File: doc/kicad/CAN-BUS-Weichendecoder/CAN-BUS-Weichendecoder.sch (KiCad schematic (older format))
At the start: 53 parts, among them J1 250-1404, J1001 Conn_01x02_Female, J1003 Conn_01x07_Female, J11 250-1406, J12 Wago 250-1406, J13 Wago 250-1406, J14 Wago 250-1406, J15 Wago 250-1406, J2 250-1404, J22 J22, J23 J22, J3 250-1404, J31 12V DC, J4 250-1404, J41 2604-1102, J5 250-1404, U1 Arduino_Nano, U10 TSR_1-2450, U1001 6N136, U2 ULN2803A, U3 ULN2803A, U4 PCF8574, U5 PCF8574, U6 PCF8574, U7 ULN2803A, U8 ULN2803A, U9 ULN2803A

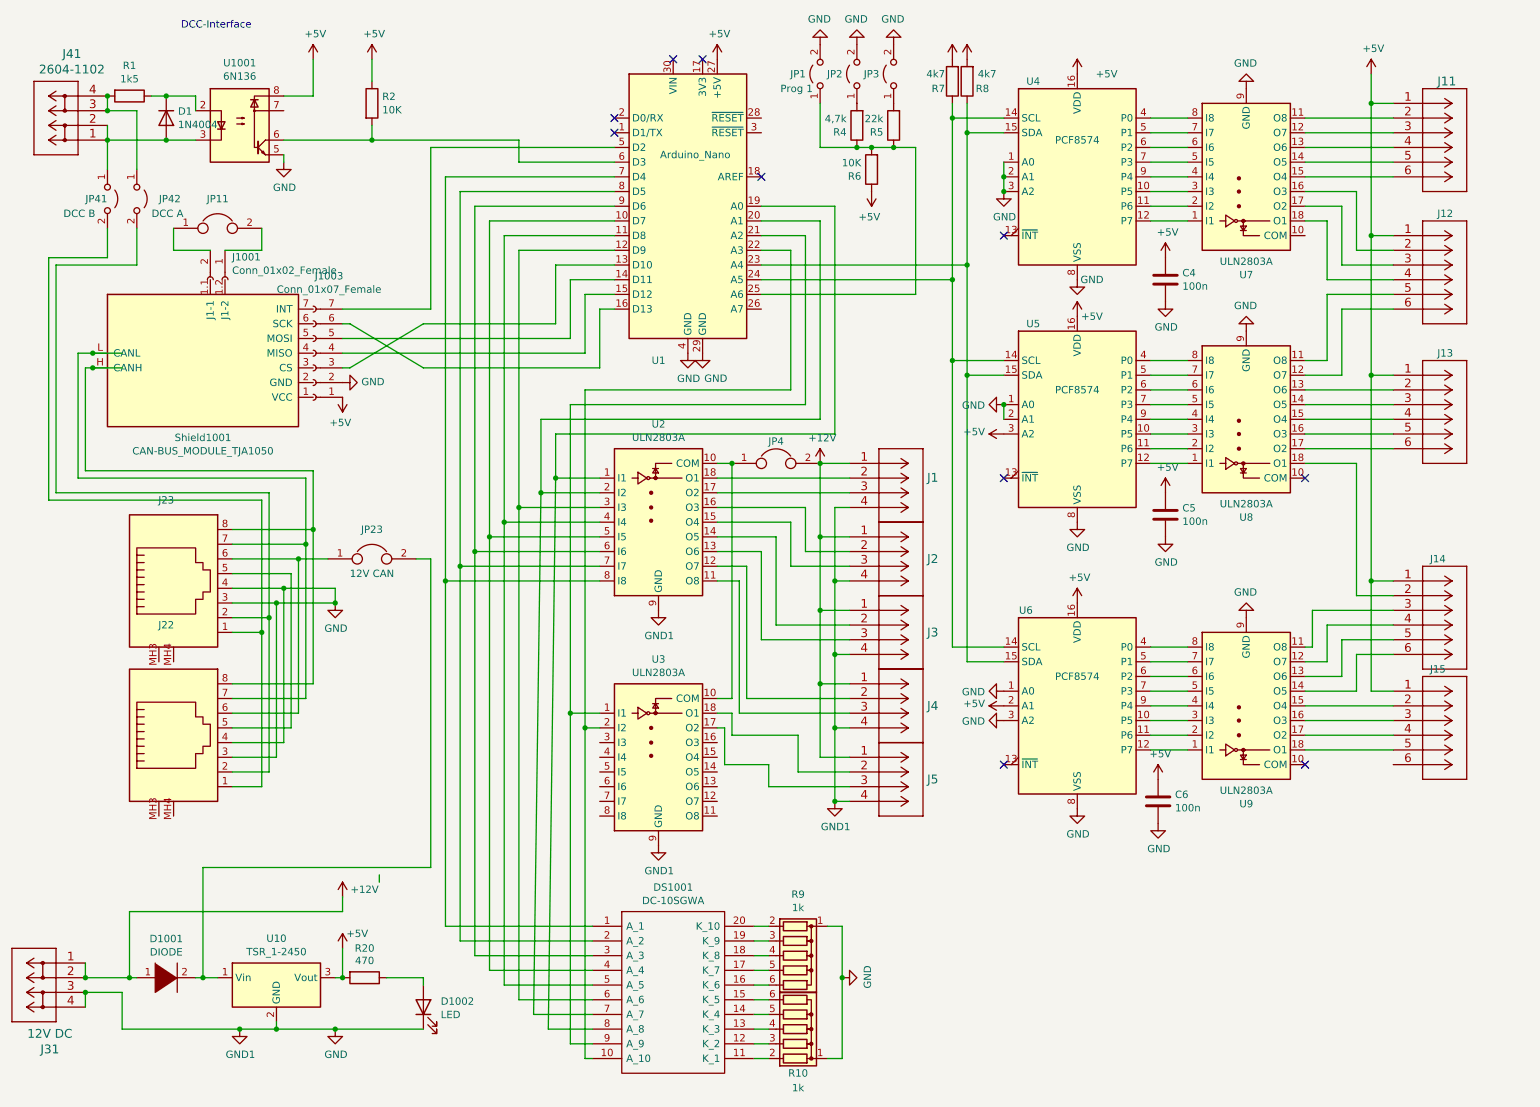
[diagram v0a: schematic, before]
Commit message: verbessert
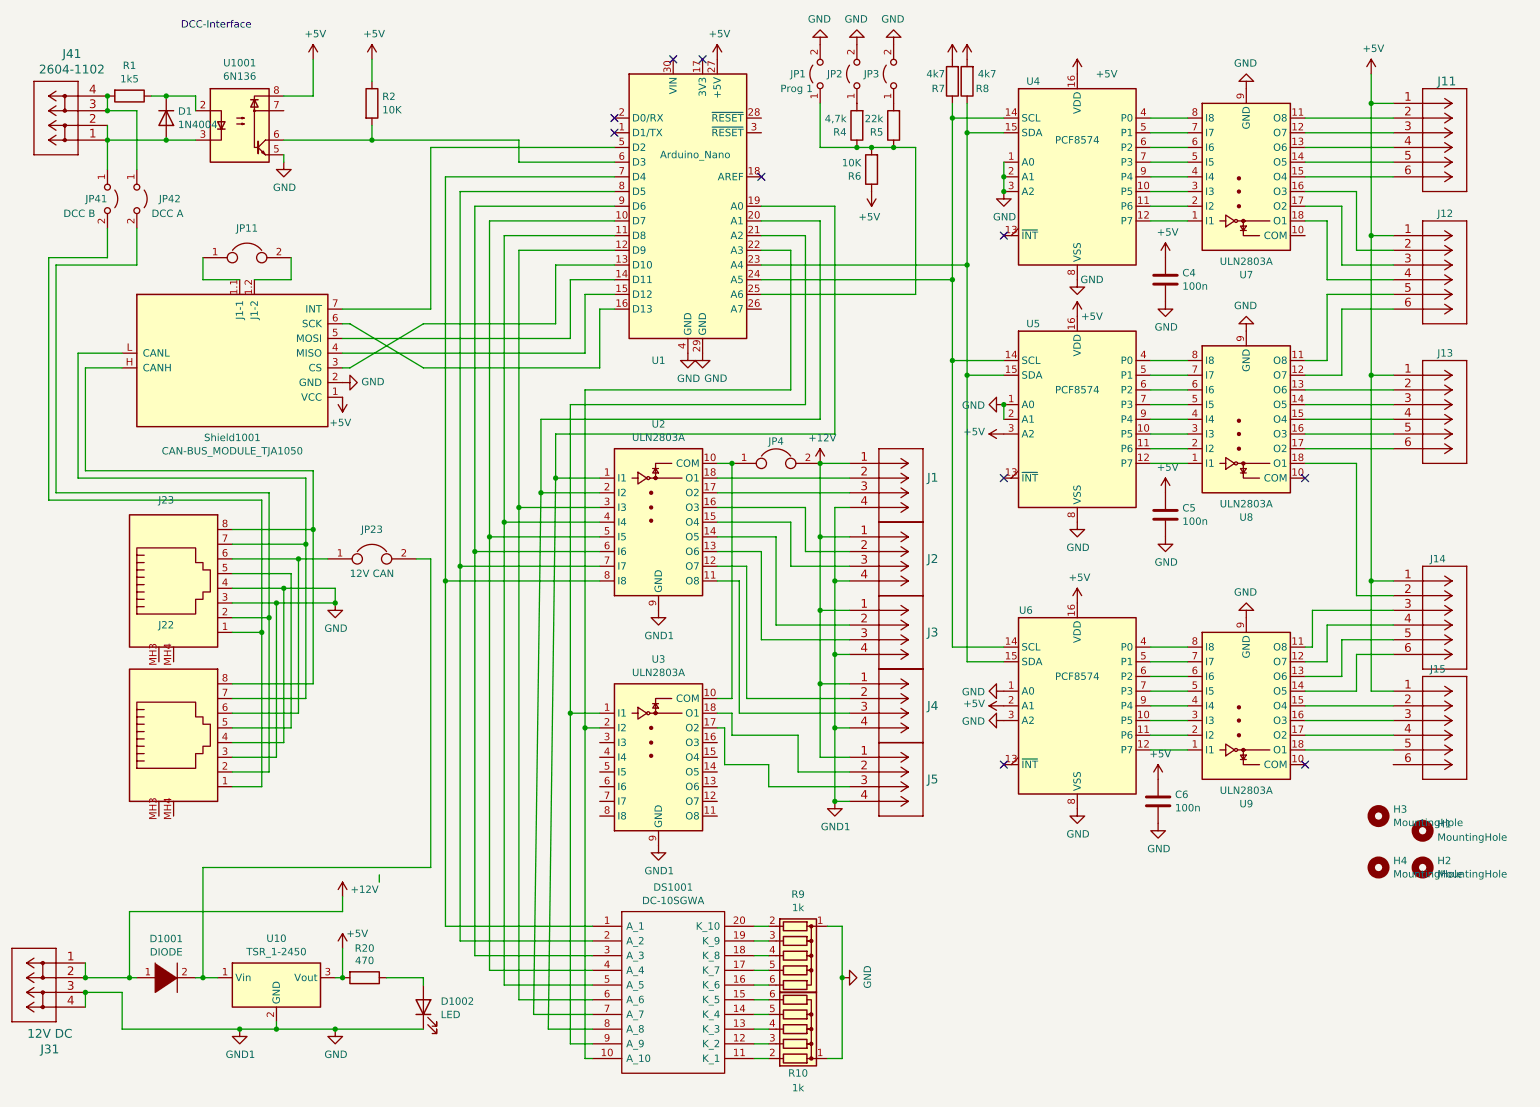
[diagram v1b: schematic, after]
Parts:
- removed J1001: Conn_01x02_Female, Pin_Headers:Pin_Header_Straight_1x02_Pitch2.54mm, symbol Connector:Conn_01x02_Female
- removed J1003: Conn_01x07_Female, Pin_Headers:Pin_Header_Straight_1x07_Pitch2.54mm, symbol Connector:Conn_01x07_Female
- added H1, H2, H3, H4: MountingHole, Mounting_Holes:MountingHole_3.2mm_M3, symbol Mechanical:MountingHole
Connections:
- net +5V: now also Shield1001.1 (VCC)
- net GND: now also Shield1001.2 (GND)
- net at U1.13 (D10): now also Shield1001.3 (CS)
- net at U1.14 (D11): now also Shield1001.5 (MOSI)
- net at U1.15 (D12): now also Shield1001.4 (MISO)
- net at U1.16 (D13): now also Shield1001.6 (SCK)
- net at U1.5 (D2): now also Shield1001.7 (INT)
- net at Shield1001.1.1 (J1-1): now also JP11.1
- net at Shield1001.1.2 (J1-2): now also JP11.2
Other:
- moved on the sheet: JP11, Shield1001
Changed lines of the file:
@@
 L CAN-BUS-MODULE-TJA1050:CAN-BUS_MODULE_TJA1050 Shield1001
 U 1 1 60585225
-P 2000 2650
-F 0 "Shield1001" H 1950 1975 50  0000 C CNN
-F 1 "CAN-BUS_MODULE_TJA1050" H 1950 1884 50  0000 C CNN
-F 2 "CAN-BUS-MODULE:MCP2515_CAN_MODULE_BY0-10" H 2000 2650 50  0001 C CIN
-F 3 "" H 2000 2650 50  0001 C CNN
-	1    2000 2650
+P 2200 2650
+F 0 "Shield1001" H 2150 1975 50  0000 C CNN
+F 1 "CAN-BUS_MODULE_TJA1050" H 2150 1884 50  0000 C CNN
+F 2 "CAN-BUS-MODULE:MCP2515_CAN_MODULE_BY0-10" H 2200 2650 50  0001 C CIN
+F 3 "" H 2200 2650 50  0001 C CNN
+	1    2200 2650
 	1    0    0    -1
 $EndComp
@@
 	2700 5000 2150 5000
 Wire Wire Line
-	1400 2850 1200 2850
+	1400 2850 1150 2850
 Wire Wire Line
 	1150 2850 1150 3550
 Wire Wire Line
-	1400 2750 1200 2750
+	1400 2750 1100 2750
 Wire Wire Line
 	1100 2750 1100 3600
 Wire Wire Line
 	4750 1750 3800 1750
-Connection ~ 1200 2850
-Wire Wire Line
-	1200 2850 1150 2850
-Connection ~ 1200 2750
-$Comp
-L Connector:Conn_01x07_Female J1003
-U 1 1 60962CDF
-P 2700 2750
-F 0 "J1003" H 2592 2225 50  0000 C CNN
-F 1 "Conn_01x07_Female" H 2592 2316 50  0000 C CNN
-F 2 "Pin_Headers:Pin_Header_Straight_1x07_Pitch2.54mm" H 2700 2750 50  0001 C CNN
-F 3 "~" H 2700 2750 50  0001 C CNN
-	1    2700 2750
-	-1   0    0    1
-$EndComp
-Wire Wire Line
-	1100 2750 1200 2750
 $Comp
 L Isolator:6N136 U1001
@@
 	1150 7200 1150 7100
 Connection ~ 1150 7100
-$Comp
-L Connector:Conn_01x02_Female J1001
-U 1 1 61A1EF28
-P 2100 2250
-F 0 "J1001" V 1946 2298 50  0000 L CNN
-F 1 "Conn_01x02_Female" V 2037 2298 50  0000 L CNN
-F 2 "Pin_Headers:Pin_Header_Straight_1x02_Pitch2.54mm" H 2100 2250 50  0001 C CNN
-F 3 "~" H 2100 2250 50  0001 C CNN
-	1    2100 2250
-	0    1    1    0
-$EndComp
-Wire Wire Line
-	1750 1900 1750 2050
-Wire Wire Line
-	1750 2050 2000 2050
-Wire Wire Line
-	2100 2050 2350 2050
-Wire Wire Line
-	2350 2050 2350 1900
+Wire Wire Line
+	1950 2100 1950 2250
+Wire Wire Line
+	1950 2250 2200 2250
+Wire Wire Line
+	2550 2250 2550 2100
 $Comp
 L Device:Jumper JP11
 U 1 1 61A202D7
-P 2050 1900
-F 0 "JP11" H 2050 2100 50  0000 C CNN
-F 1 "Jumper" H 2050 2073 50  0001 C CNN
-F 2 "Pin_Headers:Pin_Header_Straight_1x02_Pitch2.54mm" H 2050 1900 50  0001 C CNN
-F 3 "~" H 2050 1900 50  0001 C CNN
-	1    2050 1900
+P 2250 2100
+F 0 "JP11" H 2250 2300 50  0000 C CNN
+F 1 "Jumper" H 2250 2273 50  0001 C CNN
+F 2 "Pin_Headers:Pin_Header_Straight_1x02_Pitch2.54mm" H 2250 2100 50  0001 C CNN
+F 3 "~" H 2250 2100 50  0001 C CNN
+	1    2250 2100
 	1    0    0    -1
 $EndComp
@@
 	3450 7350 2850 7350
 Connection ~ 2850 7350
+Wire Wire Line
+	2300 2250 2550 2250
+$Comp
+L Mechanical:MountingHole H1
+U 1 1 622C717E
+P 10250 6000
+F 0 "H1" H 10350 6046 50  0000 L CNN
+F 1 "MountingHole" H 10350 5955 50  0000 L CNN
+F 2 "Mounting_Holes:MountingHole_3.2mm_M3" H 10250 6000 50  0001 C CNN
+F 3 "~" H 10250 6000 50  0001 C CNN
+	1    10250 6000
+	1    0    0    -1
+$EndComp
+$Comp
+L Mechanical:MountingHole H2
+U 1 1 622C9821
+P 10250 6250
+F 0 "H2" H 10350 6296 50  0000 L CNN
+F 1 "MountingHole" H 10350 6205 50  0000 L CNN
+F 2 "Mounting_Holes:MountingHole_3.2mm_M3" H 10250 6250 50  0001 C CNN
+F 3 "~" H 10250 6250 50  0001 C CNN
+	1    10250 6250
+	1    0    0    -1
+$EndComp
+$Comp
+L Mechanical:MountingHole H4
+U 1 1 62312DA2
+P 9950 6250
+F 0 "H4" H 10050 6296 50  0000 L CNN
+F 1 "MountingHole" H 10050 6205 50  0000 L CNN
+F 2 "Mounting_Holes:MountingHole_3.2mm_M3" H 9950 6250 50  0001 C CNN
+F 3 "~" H 9950 6250 50  0001 C CNN
+	1    9950 6250
+	1    0    0    -1
+$EndComp
+$Comp
+L Mechanical:MountingHole H3
+U 1 1 62380421
+P 9950 5900
+F 0 "H3" H 10050 5946 50  0000 L CNN
+F 1 "MountingHole" H 10050 5855 50  0000 L CNN
+F 2 "Mounting_Holes:MountingHole_3.2mm_M3" H 9950 5900 50  0001 C CNN
+F 3 "~" H 9950 5900 50  0001 C CNN
+	1    9950 5900
+	1    0    0    -1
+$EndComp
 $EndSCHEMATC
